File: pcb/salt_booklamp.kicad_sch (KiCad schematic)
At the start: 28 parts, among them J1 USB-C31-S-RA-CS1E-BK-T/R, P1 PIC-TC2050-IDC, U1 PIC16F15213-I/SN, U2 BQ21040DBVR, U3 TPS61158DRVR

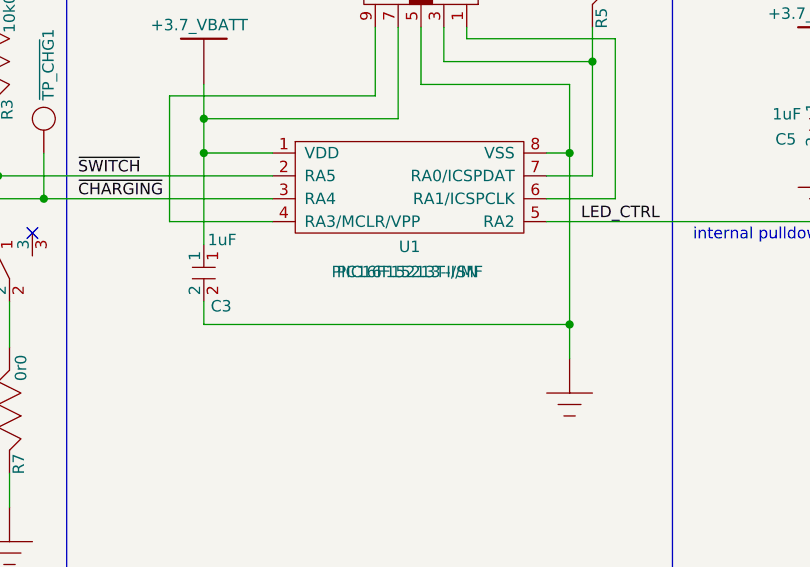
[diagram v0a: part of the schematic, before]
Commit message: Placement work
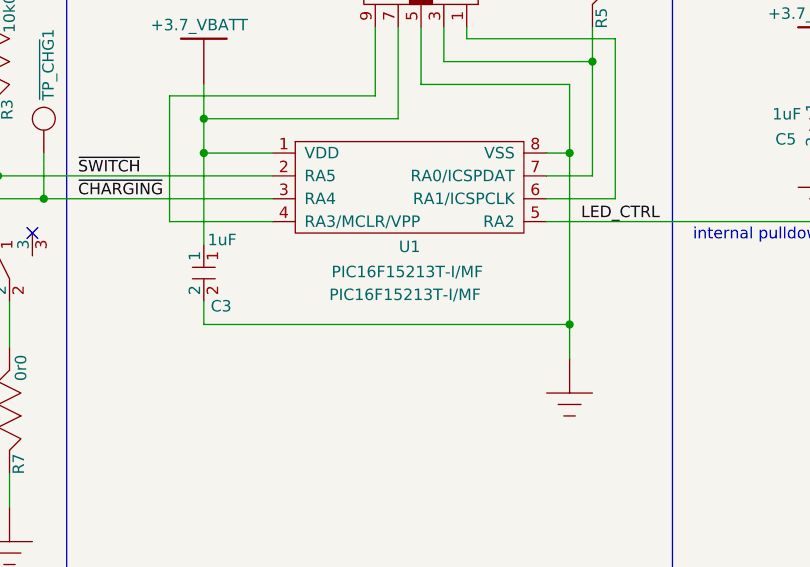
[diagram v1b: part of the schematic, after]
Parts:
- U1: value PIC16F15213-I/SN -> PIC16F15213T-I/MF
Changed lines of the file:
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@@
 			"AAAAAAAAAAAAAAAAAAAAAAAAAAAAAAAAAAAAAAAAAAAAAAAAAAAAAAAAAAAAAAAAAAAAAAAAAAAA"
 			"AAAAAAAAAAAAAAAAAAAAAAAAAAAAAAAAAAAAAAAAAAAAAAAAAAAAAAAAAAAAAAAAAAAAAAAAAAAA"
+			"AAAAAAAAAAAAAAAAAAAAAAAAAAAAAAAAAAAAAAAAAAAAAAAAAAAAAAAAAAAAAAAAAAAAAAAAAAAA"
+			"AAAAAAAAAAAAAAAAAAAAAAAAAAAAAAAAAAAAAAAAAAAAAAAAAAAAAAAAAAAAAAAAAAAAAAAAAAAA"
+			"AAAAAAAAAAAAAAAAAAAAAAAAAAAAAAAAAAAAAAAAAAAAAAAAAAAAAAAAAAAAAAAAAAAAAAAAAAAA"
+			"AAAAAAAAAAAAAAAAAAAAAAAAAAAAAAAAAAAAAAAAAAAAAAAAAAAAAAAAAAAAAAAAAAAAAAAAAAAA"
+			"AAAAAAAAAAAAAAAAAAAAAAAAAAAAAAAAAAAAAAAAAAAAAAAAAAAAAAAAAAAAAAAAAAAAAAAAAAAA"
+			"AAAAAAAAAAAAAAAAAAAAAAAAAAAAAAAAAAAAAAAAAAAAAAAAAAAAAAAAAAAAAAAAAAAAAAAAAAAA"
+			"AAAAAAAAAAAAAAAAAAAAAAAAAAAAAAAAAAAAAAAAAAAAAAAAAAAAAAAAAAAAAAAAAAAAAAAAAAAA"
+			"AAAAAAAAAAAAAAAAAAAAAAAAAAAAAAAAAAAAAAAAAAAAAAAAAAAAAAAAAAAAAAAAAAAAAAAAAAAA"
+			"AAAAAAAAAAAAAAAAAAAAAAAAAAAAAAAAAAAAAAAAAAAAAAAAAAAAAAAAAAAAAAAAAAAAAAAAAAAA"
+			"AAAAAAAAAAAAAAAAAAAAAAAAAAAAAAAAAAAAAAAAAAAAAAAAAAAAAAAAAAAAAAAAAAAAAAAAAAAA"
+			"AAAAAAAAAAAAAAAAAAAAAAAAAAAAAAAAAAAAAAAAAAAAAAAAAAAAAAAAAAAAAAAAAAAAAAAAAAAA"
+			"AAAAAAAAAAAAAAAAAAAAAAAAAAAAAAAAAAAAAAAAAAAAAAAAAAAAAAAAAAAAAAAAAAAAAAAAAAAA"
+			"AAAAAAAAAAAAAAAAAAAAAAAAAAAAAAAAAAAAAAAAAAAAAAAAAAAAAAAAAAAAAAAAAAAAAAAAAAAA"
+			"AAAAAAAAAAAAAAAAAAAAAAAAAAAAAAAAAAAAAAAAAAAAAAAAAAAAAAAAAAAAAAAAAAAAAAAAAAAA"
+			"AAAAAAAAAAAAAAAAAAAAAAAAAAAAAAAAAAAAAAAAAAAAAAAAAAAAAAAAAAAAAAAAAAAAAAAAAAAA"
+			"AAAAAAAAAAAAAAAAAAAAAAAAAAAAAAAAAAAAAAAAAAAAAAAAAAAAAAAAAAAAAAAAAAAAAAAAAAAA"
+			"AAAAAAAAAAAAAAAAAAAAAAAAAAAAAAAAAAAAAAAAAAAAAAAAAAAAAAAAAAAAAAAAAAAAAAAAAAAA"
+			"AAAAAAAAAAAAAAAAAAAAAAAAAAAAAAAAAAAAAAAAAAAAAAAAAAAAAAAAAAAAAAAAAAAAAAAAAAAA"
 			"AAAAAAAAAA=="
 		)
@@
 			)
 		)
-		(property "Value" "PIC16F15213-I/SN"
-			(at 173.736 119.888 0)
+		(property "Value" "PIC16F15213T-I/MF"
+			(at 173.482 122.428 0)
 			(effects
 				(font
@@
 			)
 		)
-		(property "Description" "PIC PIC® 16F, Functional Safety (FuSa) Microcontroller IC 8-Bit 32MHz 3.5KB (2K x 14) FLASH 8-SOIC"
+		(property "Description" "PIC PIC® 16F, Functional Safety (FuSa) Microcontroller IC 8-Bit 32MHz 3.5KB (2K x 14) FLASH 8-DFN (3x3)"
 			(at 173.99 110.49 0)
 			(effects
